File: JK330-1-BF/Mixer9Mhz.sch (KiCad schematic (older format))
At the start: 12 parts

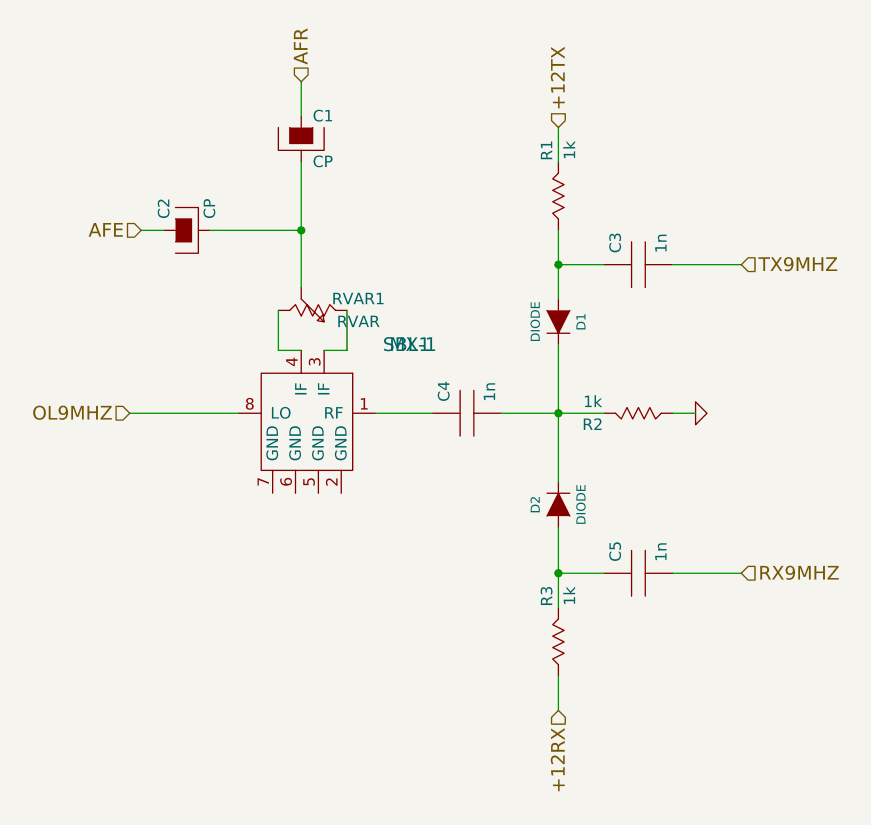
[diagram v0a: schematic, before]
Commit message: MAJ  composants
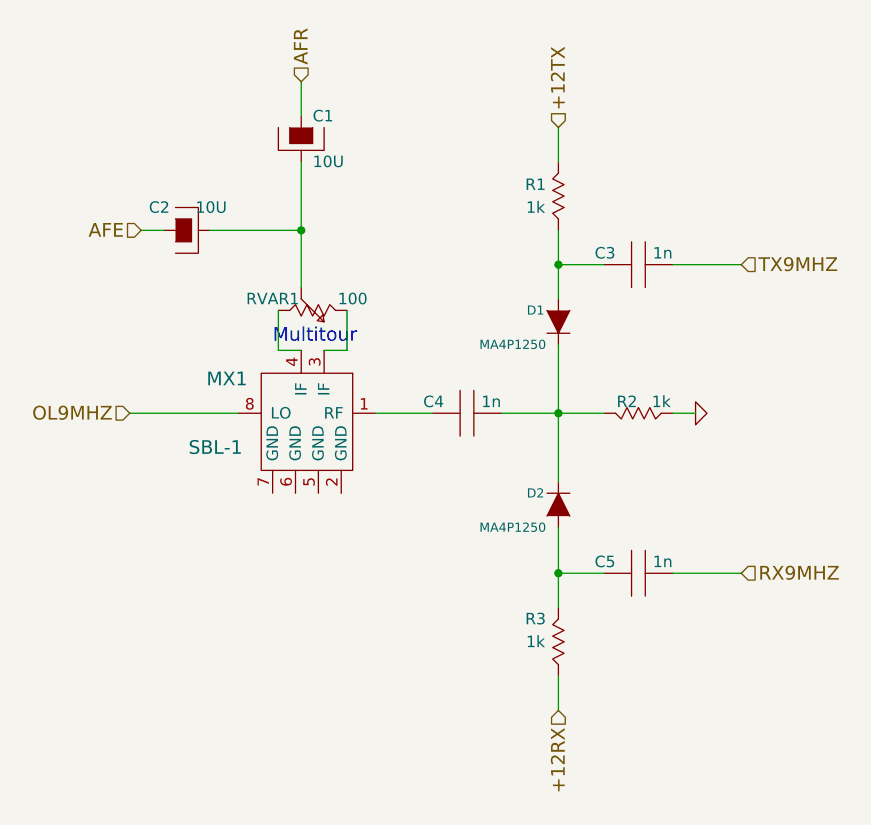
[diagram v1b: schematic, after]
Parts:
- C1, C2: value CP -> 10U
- D1, D2: value DIODE -> MA4P1250
- RVAR1: value RVAR -> 100
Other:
- note added: "Multitour"
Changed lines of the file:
@@
-EESchema Schematic File Version 2  date 2013-03-25 22:18:17
+EESchema Schematic File Version 2  date 29/04/2013 22:12:34
 LIBS:power
 LIBS:CEN-SCHEMA
@@
 Sheet 2 6
 Title ""
-Date "25 mar 2013"
+Date "29 apr 2013"
 Rev ""
 Comp ""
@@
 P 5025 2600
 F 0 "C1" H 5075 2700 50  0000 L CNN
-F 1 "CP" H 5075 2500 50  0000 L CNN
+F 1 "10U" H 5075 2500 50  0000 L CNN
 F 2 "" H 5025 2600 60  0001 C CNN
 F 3 "" H 5025 2600 60  0001 C CNN
@@
 U 1 1 514E2FF7
 P 4525 3000
-F 0 "C2" H 4575 3100 50  0000 L CNN
-F 1 "CP" H 4575 2900 50  0000 L CNN
+F 0 "C2" V 4625 3075 50  0000 L CNN
+F 1 "10U" V 4625 2825 50  0000 L CNN
 F 2 "" H 4525 3000 60  0001 C CNN
 F 3 "" H 4525 3000 60  0001 C CNN
@@
 U 1 1 514E2DD7
 P 5175 3350
-F 0 "RVAR1" V 5125 3450 50  0000 C CNN
-F 1 "RVAR" V 5225 3450 50  0000 C CNN
+F 0 "RVAR1" V 5125 3075 50  0000 C CNN
+F 1 "100" V 5125 3425 50  0000 C CNN
 F 2 "" H 5175 3350 60  0001 C CNN
 F 3 "" H 5175 3350 60  0001 C CNN
@@
 U 1 1 514E2D7C
 P 6150 4700
-F 0 "R3" V 6100 4800 50  0000 C CNN
-F 1 "1k" V 6200 4800 50  0000 C CNN
+F 0 "R3" H 6050 4700 50  0000 C CNN
+F 1 "1k" H 6050 4600 50  0000 C CNN
 F 2 "" H 6150 4700 60  0001 C CNN
 F 3 "" H 6150 4700 60  0001 C CNN
@@
 U 1 1 514E2D6E
 P 6150 2750
-F 0 "R1" V 6100 2850 50  0000 C CNN
-F 1 "1k" V 6200 2850 50  0000 C CNN
+F 0 "R1" H 6050 2700 50  0000 C CNN
+F 1 "1k" H 6050 2600 50  0000 C CNN
 F 2 "" H 6150 2750 60  0001 C CNN
 F 3 "" H 6150 2750 60  0001 C CNN
@@
 U 1 1 514E2D5C
 P 5750 3800
-F 0 "C4" H 5800 3900 50  0000 L CNN
-F 1 "1n" H 5800 3700 50  0000 L CNN
+F 0 "C4" V 5800 3900 50  0000 L CNN
+F 1 "1n" V 5800 3650 50  0000 L CNN
 F 2 "" H 5750 3800 60  0001 C CNN
 F 3 "" H 5750 3800 60  0001 C CNN
@@
 U 1 1 514E2D51
 P 5500 3500
-F 0 "MX1" H 5500 3500 60  0000 C CNN
-F 1 "SBL-1" H 5500 3500 60  0000 C CNN
+F 0 "MX1" H 6300 3350 60  0000 C CNN
+F 1 "SBL-1" H 6350 3050 60  0000 C CNN
 F 2 "" H 5500 3500 60  0001 C CNN
 F 3 "" H 5500 3500 60  0001 C CNN
@@
 U 1 1 514E29B3
 P 6400 3800
-F 0 "R2" V 6350 3900 50  0000 C CNN
-F 1 "1k" V 6450 3900 50  0000 C CNN
+F 0 "R2" V 6450 3750 50  0000 C CNN
+F 1 "1k" V 6450 3600 50  0000 C CNN
 F 2 "" H 6400 3800 60  0001 C CNN
 F 3 "" H 6400 3800 60  0001 C CNN
@@
 U 1 1 514E299B
 P 6500 4500
-F 0 "C5" H 6550 4600 50  0000 L CNN
-F 1 "1n" H 6550 4400 50  0000 L CNN
+F 0 "C5" V 6550 4600 50  0000 L CNN
+F 1 "1n" V 6550 4350 50  0000 L CNN
 F 2 "" H 6500 4500 60  0001 C CNN
 F 3 "" H 6500 4500 60  0001 C CNN
@@
 U 1 1 514E2995
 P 6500 3150
-F 0 "C3" H 6550 3250 50  0000 L CNN
-F 1 "1n" H 6550 3050 50  0000 L CNN
+F 0 "C3" V 6550 3250 50  0000 L CNN
+F 1 "1n" V 6550 3000 50  0000 L CNN
 F 2 "" H 6500 3150 60  0001 C CNN
 F 3 "" H 6500 3150 60  0001 C CNN
@@
 U 1 1 514E2901
 P 6150 3400
-F 0 "D1" H 6150 3500 40  0000 C CNN
-F 1 "DIODE" H 6150 3300 40  0000 C CNN
+F 0 "D1" V 6100 3300 40  0000 C CNN
+F 1 "MA4P1250" V 6250 3200 40  0000 C CNN
 F 2 "" H 6150 3400 60  0001 C CNN
 F 3 "" H 6150 3400 60  0001 C CNN
@@
 U 1 1 514E28F2
 P 6150 4200
-F 0 "D2" H 6150 4300 40  0000 C CNN
-F 1 "DIODE" H 6150 4100 40  0000 C CNN
+F 0 "D2" V 6200 4300 40  0000 C CNN
+F 1 "MA4P1250" V 6050 4400 40  0000 C CNN
 F 2 "" H 6150 4200 60  0001 C CNN
 F 3 "" H 6150 4200 60  0001 C CNN
@@
 	0    -1   -1   0
 $EndComp
+Text Notes 4900 3500 0    60   ~ 0
+Multitour
 $EndSCHEMATC
